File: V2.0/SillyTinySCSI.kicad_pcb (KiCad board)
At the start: 4 copper layers, 53.5 x 25 mm, 61 parts, among them J1 DB25_Plug, J2 Micro_SD_Card_Det1, U1 74LVT125, U2 74LVT245, U3 74LVT125, U4 74LVT245, U5 TLV75728PDBVR, U6 Pico W

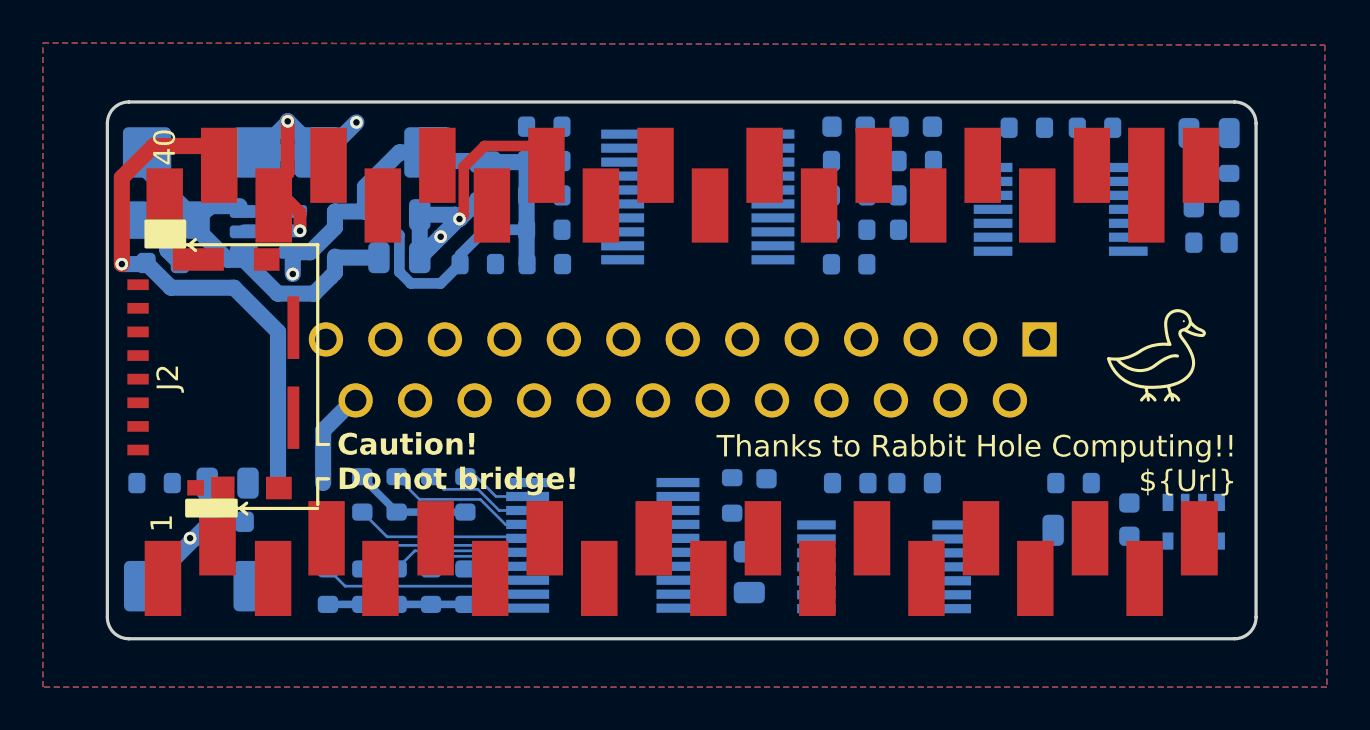
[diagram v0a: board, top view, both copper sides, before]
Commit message: routing and drc 1
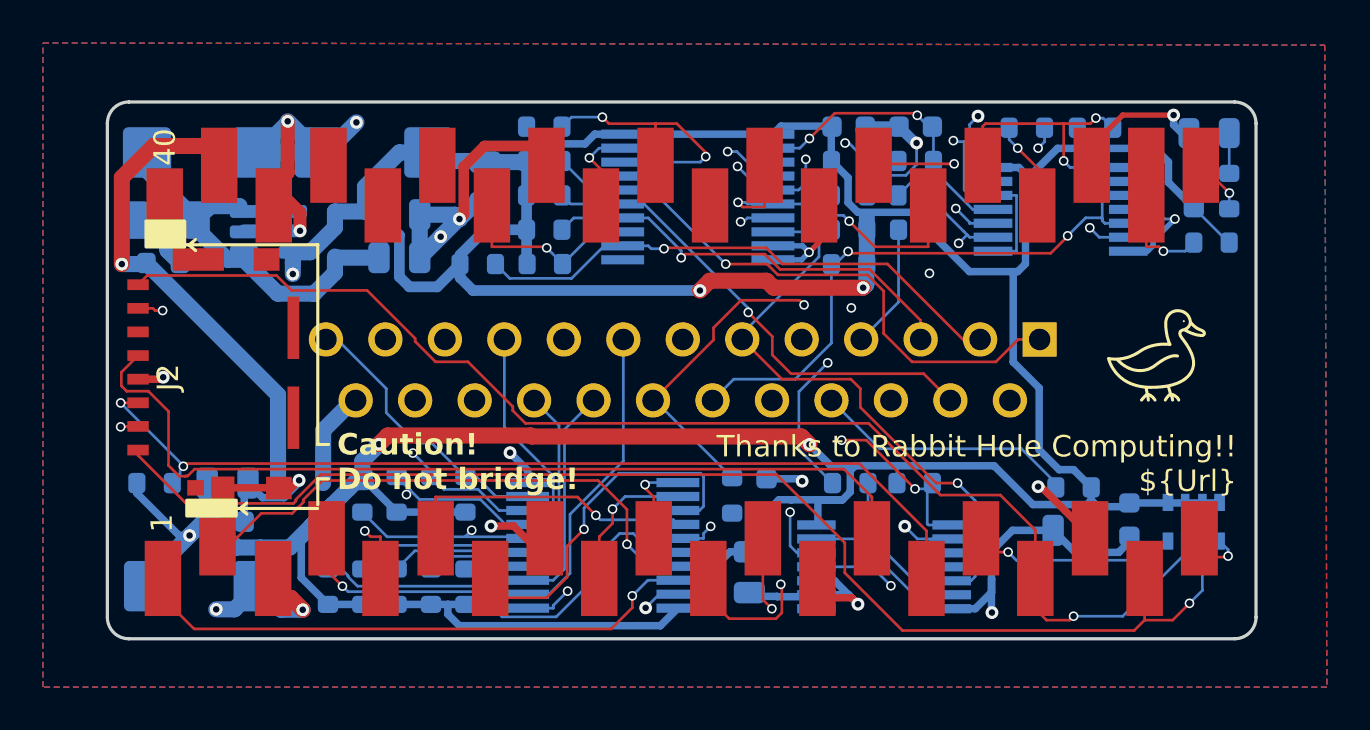
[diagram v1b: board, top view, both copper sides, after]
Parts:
- moved R13 0.20 mm to (153.0, 68.2)
- turned C2 to 180 degrees
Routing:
- net +2V8: track 63.2 -> 251.6 mm, vias 2 -> 7
- net GND: track 36.5 -> 132.7 mm, vias 5 -> 24
- net /cpu/SDIO_D0: track 0.00 -> 63.6 mm, vias 0 -> 2
- net /cpu/SDIO_D3: track 0.00 -> 62.6 mm, vias 0 -> 2
- net /cpu/SDIO_D2: track 0.00 -> 59.3 mm, vias 0 -> 1
- net /cpu/SDIO_D1: track 0.00 -> 59.3 mm, vias 0 -> 1
- net /cpu/SDIO_CMD: track 0.00 -> 44.9 mm, vias 0 -> 2
- net /cpu/SDIO_CLK: track 0.00 -> 43.4 mm
- net ~{DATA_DIR}: track 10.1 -> 48.4 mm, vias 0 -> 3
- net ~{SCSI_DBP}: track 0.00 -> 37.9 mm, vias 0 -> 2
- net ~{DBGLOG}: track 0.00 -> 30.5 mm, vias 0 -> 2
- net ~{OUT_BSY}: track 0.00 -> 29.8 mm, vias 0 -> 3
- net ~{IN_RST}: track 0.00 -> 29.4 mm, vias 0 -> 2
- net ~{GPIO_DBP}: track 0.00 -> 28.6 mm, vias 0 -> 2
- net ~{SCSI_REQ}: track 0.00 -> 27.7 mm, vias 0 -> 1
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
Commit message: sync up
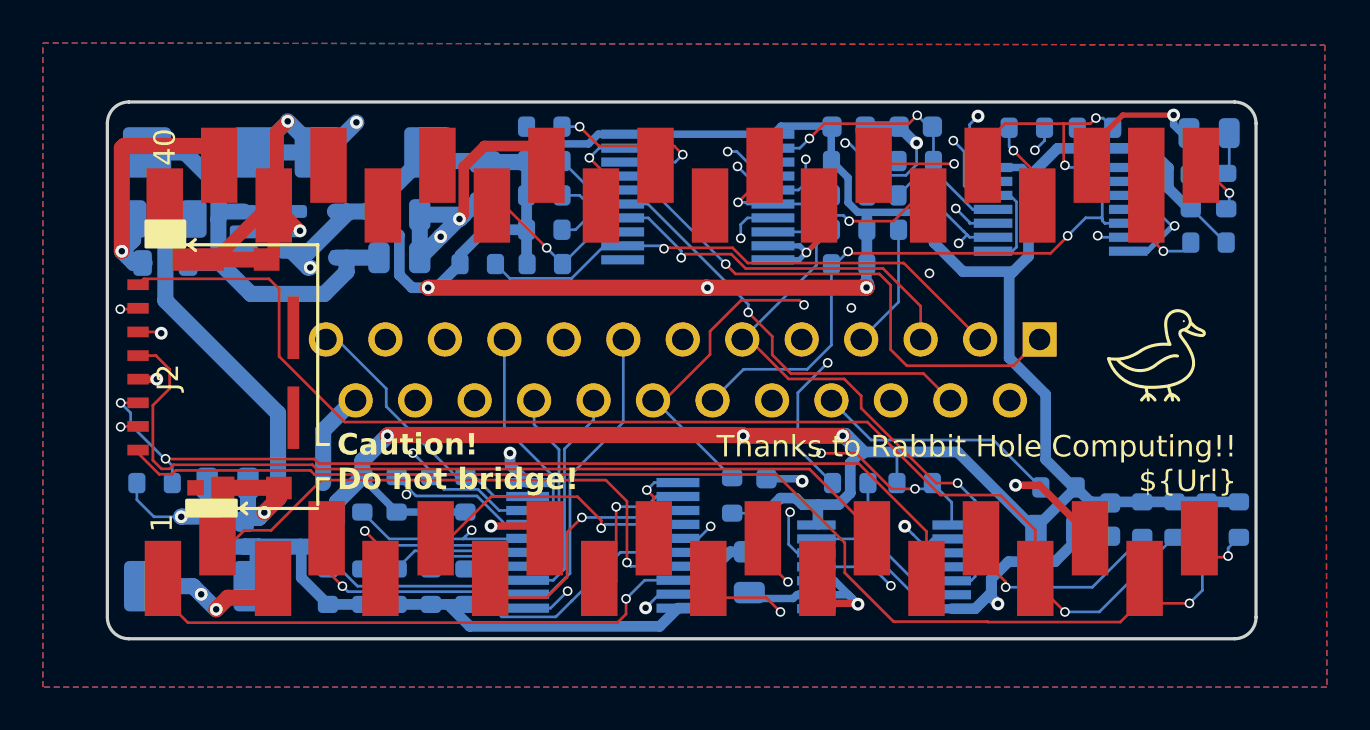
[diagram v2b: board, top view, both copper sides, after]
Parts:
- removed RN3: 4k7, Resistor_SMD:R_Array_Convex_4x0603
- added R32: 4k7, Resistor_SMD:R_0603_1608Metric, B.Cu at (160.7, 69.7)
- added R33: 4k7, Resistor_SMD:R_0603_1608Metric, B.Cu at (159.2, 69.7)
- added R34: 4k7, Resistor_SMD:R_0603_1608Metric, B.Cu at (157.7, 69.7)
- added R35: 4k7, Resistor_SMD:R_0603_1608Metric, B.Cu at (156.2, 69.7)
- L1: footprint Inductor_SMD:L_0603_1608Metric -> Inductor_SMD:L_0805_2012Metric
- moved C4 0.90 mm to (154.7, 69.7)
- moved C3 0.80 mm to (152.2, 70.2), turned to 0 degrees
- moved R13 0.70 mm to (152.3, 68.2)
- moved F1 0.16 mm to (110.6, 55.7), turned to 180 degrees
- moved R18 0.14 mm to (159.3, 56.8)
- moved C6 0.14 mm to (158.5, 54.4)
- moved R15 0.14 mm to (160.1, 54.4)
- moved L1 0.10 mm to (110.7, 57.8)
- turned C9 to 180 degrees
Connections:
- D1 pad 1: 5V_IN -> Net-(D1-K)
- F1 pad 1: Net-(F1-Pad1) -> Net-(D1-K)
- F1 pad 2: /power/5V_REG -> +5VP
- L1 pad 1: Net-(F1-Pad1) -> /power/5V_REG
- L1 pad 2: 5V_IN -> +5VP
- U6 pad 39: 5V_IN -> +5VP
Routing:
- net +2V8: track 251.6 -> 280.4 mm, vias 7 -> 9
- net 5V_IN: track 23.0 -> 0.00 mm, vias 1 -> 0
- net Net-(D1-K): track 0.00 -> 15.2 mm
- net +5VP: track 0.00 -> 12.4 mm, vias 0 -> 1
- net ~{GPIO_DB5}: track 16.5 -> 11.7 mm
- net ~{GPIO_ACK}: track 12.8 -> 9.11 mm
- net Net-(F1-Pad1): track 3.43 -> 0.00 mm
- net /power/5V_REG: track 17.1 -> 20.5 mm
- net /cpu/SDIO_D2: track 59.3 -> 56.6 mm
- net ~{GPIO_MSG_BSY}: track 24.8 -> 22.2 mm
- net /cpu/SDIO_CLK: track 43.4 -> 41.3 mm
- net ~{GPIO_DB2}: track 20.4 -> 18.5 mm
- net ~{GPIO_ATN}: track 9.84 -> 8.07 mm
- net GND: track 132.7 -> 134.3 mm, vias 24 -> 25
- net ~{GPIO_DB4}: track 14.6 -> 13.2 mm
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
